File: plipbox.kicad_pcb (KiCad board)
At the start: 2 copper layers, 10 parts, among them P1 PWR, P2 PARALLEL_PORT, P3 RS232, U1 MAX3221, U2 ARDUINO_NANO_V3

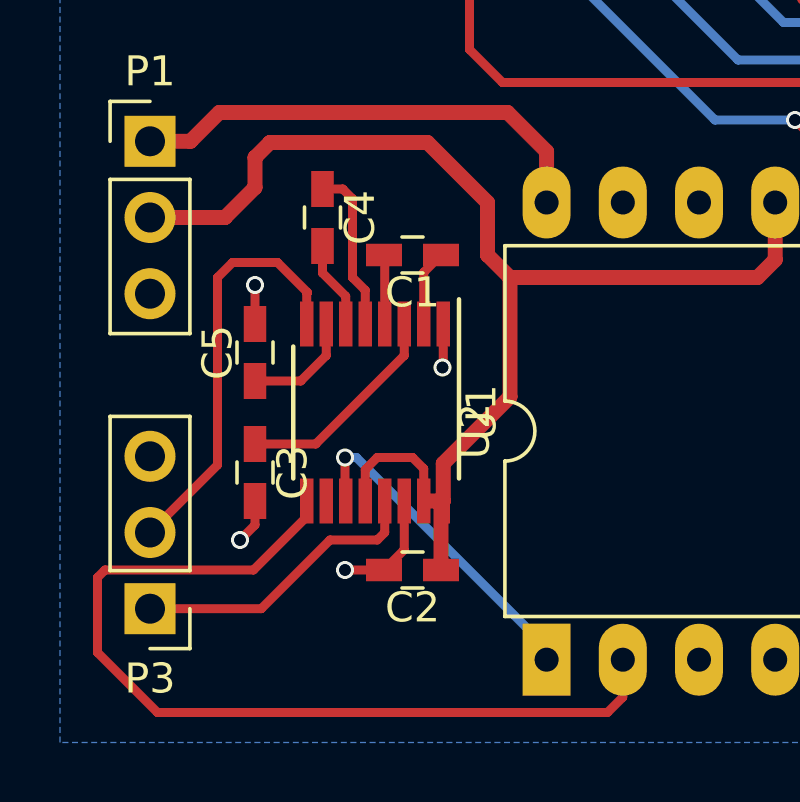
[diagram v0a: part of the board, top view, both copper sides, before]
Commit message: Silkscreen
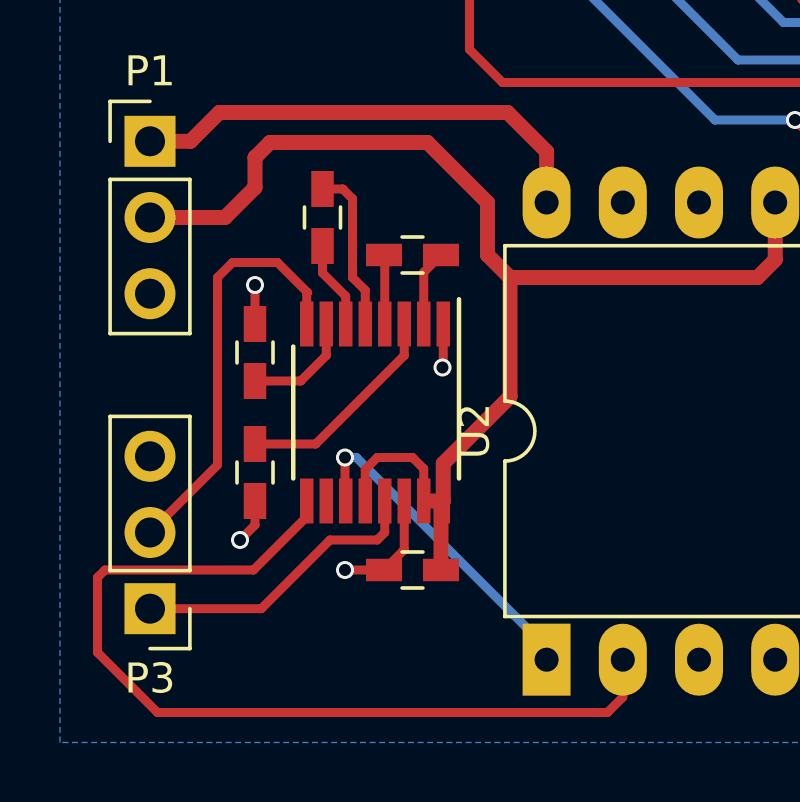
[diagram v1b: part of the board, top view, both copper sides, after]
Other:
- board text added: "1"
- board text added: "5V"
- board text added: "Arduino Nano V3"
- board text added: "DB25M"
- board text added: "GND"
- board text added: "PARALLEL PORT"
- board text added: "RS232"
- board text added: "RX"
- board text added: "TX"
- board text added: "VIN"
